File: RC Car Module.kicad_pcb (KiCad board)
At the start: 2 copper layers, 45 x 45 mm, 72 parts, among them J1 USB_C_Receptacle_USB2.0_14P, J2 Conn_01x13, J3 Conn_01x09, J4 Conn_01x02, J5 Conn_01x02, J6 Conn_01x04, J7 Conn_01x02, SW1 SW_Push, SW2 SW_Push, U1 AP62401WU-7, U2 W25Q16JVUXIQ TR, U3 RT6154AGQW, U4 TB6612FNG, U5 RP2040, Y1 12 MHz

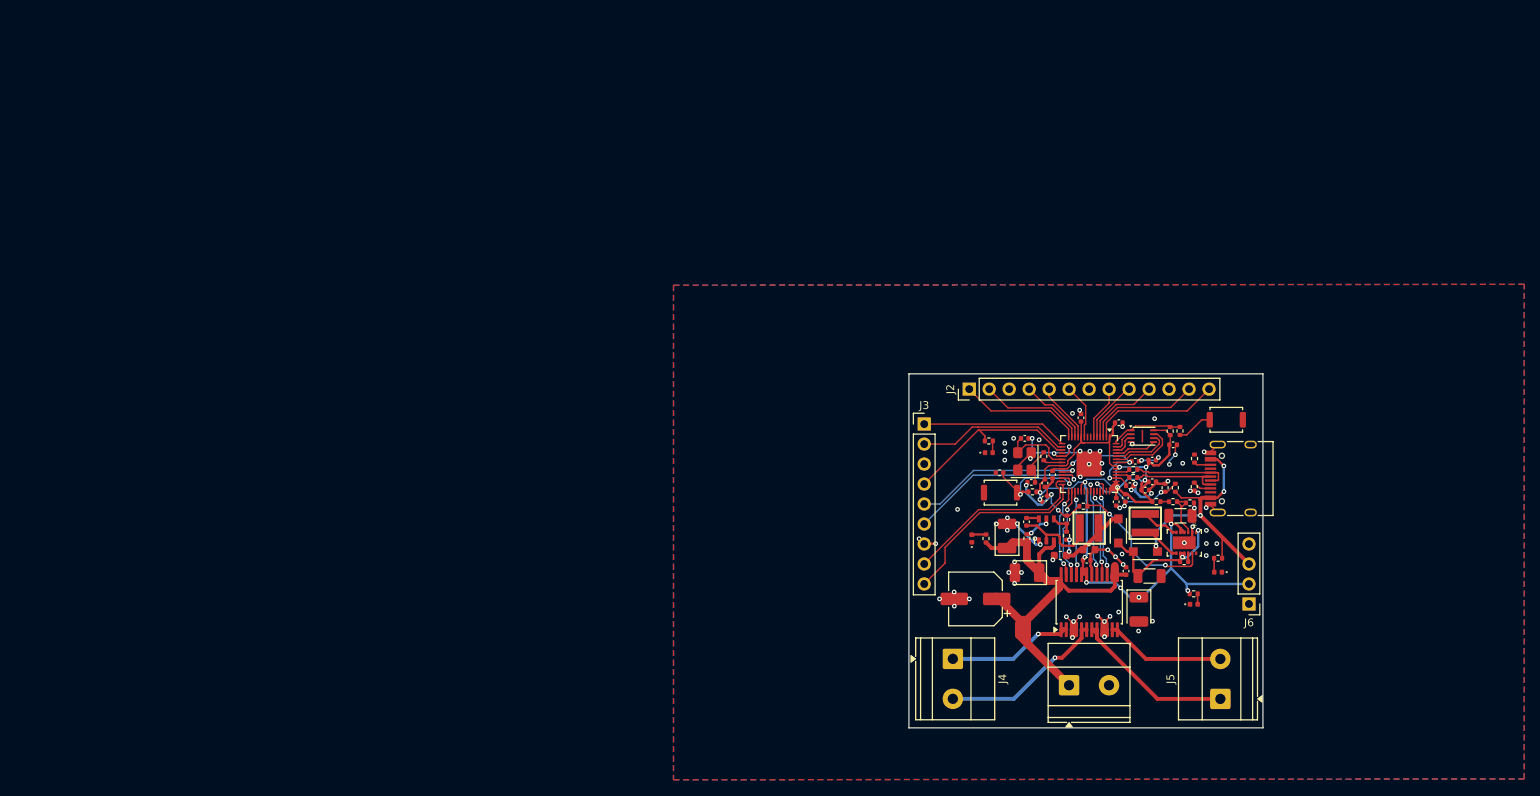
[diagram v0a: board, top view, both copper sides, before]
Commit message: Update Readme
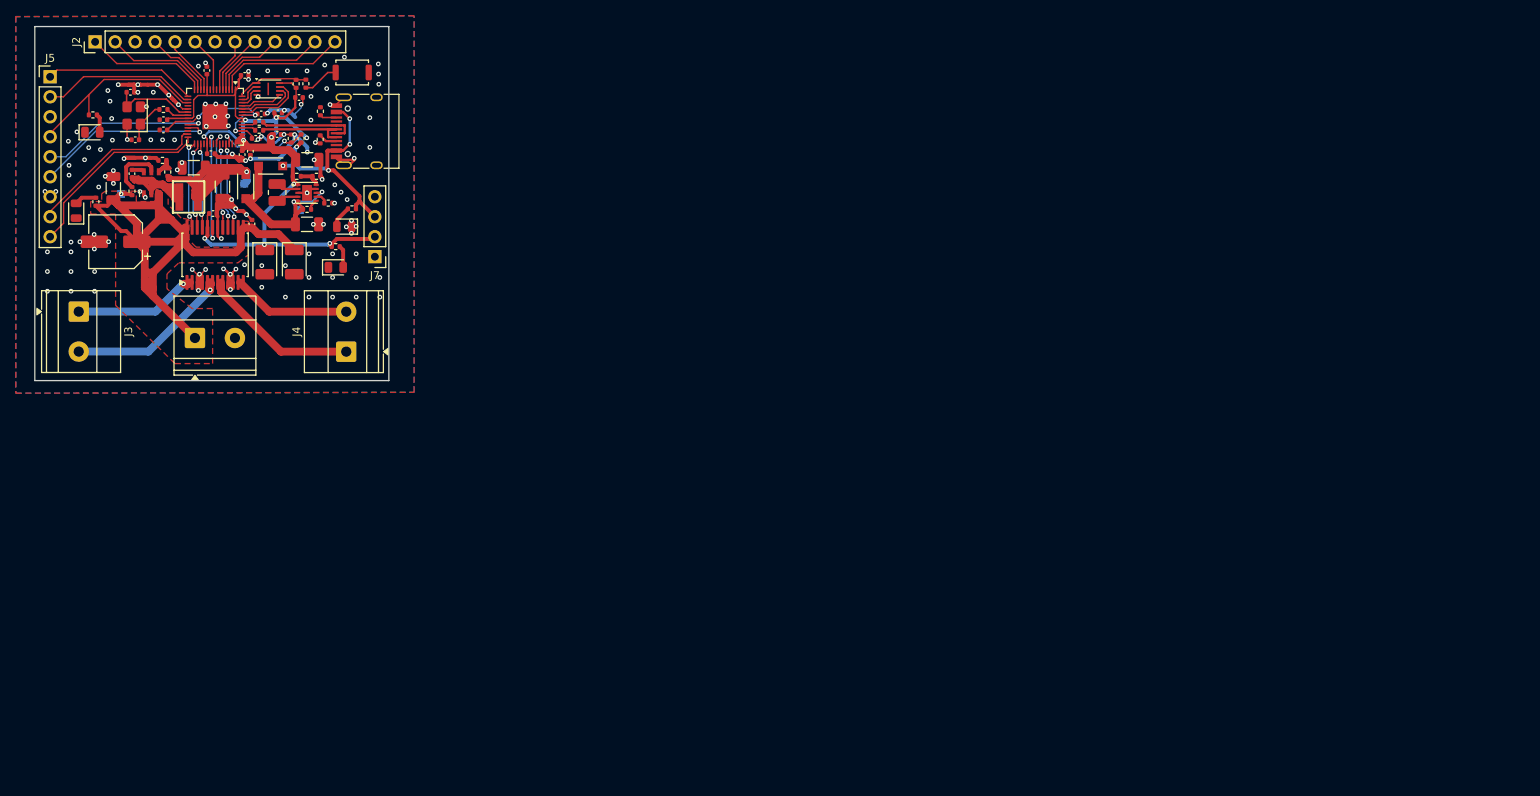
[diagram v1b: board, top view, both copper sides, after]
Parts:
- removed the C15 at (156.4, 76.3)
- removed the C23 at (155.4, 79.3)
- removed the C24 at (155.4, 77.3)
- removed C27: 0.1uF, Capacitor_SMD:C_0402_1005Metric
- removed the R12 at (171.7, 79.7)
- removed the R15 at (160.3, 80.3)
- removed the R16 at (153.8, 78.5)
- removed SW2: SW_Push, Button_Switch_SMD:SW_Push_SPST_NO_Alps_SKRK
- added C10: 1uF, Capacitor_SMD:C_0402_1005Metric, F.Cu at (55.1, 33.5)
- added C14: 0.1uF, Capacitor_SMD:C_0402_1005Metric, F.Cu at (49.4, 35.5)
- added R7: 100K, Resistor_SMD:R_0402_1005Metric, F.Cu at (61.6, 42.6)
- added TP1: TestPoint, TestPoint:TestPoint_Pad_1.0x1.0mm, B.Cu at (38.0, 40.6)
- added TP2: TestPoint, TestPoint:TestPoint_Pad_1.0x1.0mm, B.Cu at (53.7, 39.3)
- added TP3: TestPoint, TestPoint:TestPoint_Pad_1.0x1.0mm, B.Cu at (60.8, 42.7)
- C4: footprint Capacitor_Tantalum_SMD:CP_EIA-3528-15_AVX-H -> Capacitor_SMD:C_1206_3216Metric
- C6, C7: footprint Capacitor_SMD:C_0603_1608Metric -> Capacitor_SMD:C_1206_3216Metric
- C8: renamed from C9; value 47uF -> 10uF
- C9: renamed from C8; value 47uF -> 22uF
- D1, D2, D3, D4: footprint LED_SMD:LED_0402_1005Metric -> LED_SMD:LED_0805_2012Metric
- L2: footprint easyeda2kicad:IND-SMD_L4.0-W4.0_XAL4030-332MEC -> Inductor_SMD:L_1008_2520Metric
- R9: renamed from R8; value 330K -> 1.02M
- U3: value RT6154AGQW -> RT6150BGQW; footprint RP2040:QFN_4AGQW_RIT -> easyeda2kicad:WSON-10_L2.5-W2.5-P0.50-BL-EP
- moved C19 133.4 mm to (43.4, 31.2), turned to 180 degrees
- moved C11 130.9 mm to (43.4, 32.5), turned to 180 degrees
- moved C4 126.0 mm to (37.0, 39.9), turned to 90 degrees
- moved C6 123.7 mm to (47.2, 37.3), turned to 180 degrees
- moved R6 123.7 mm to (43.3, 36.3), turned to 180 degrees
- moved R2 123.2 mm to (44.0, 37.8)
- moved C13 122.1 mm to (54.5, 35.2), turned to -90 degrees
- moved U1 122.0 mm to (41.9, 39.2)
- moved R1 122.0 mm to (39.4, 40.2)
- moved C1 122.0 mm to (39.4, 38.0)
- moved L1 122.0 mm to (46.6, 41.0)
- moved C5 121.9 mm to (39.8, 33.7)
- moved C2 121.9 mm to (39.2, 27.7)
- moved 1111111111111 121.5 mm to (57.0, 37.0)
- moved Y1 121.4 mm to (39.6, 30.6)
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- renumbered 111111 to 1111111111111, 1111111 to 11111111111111, C16 to C11, C17 to C12, C18 to C13, C20 to C15, C21 to C16, C22 to C17, C25 to C20, C26 to C21, C10 to C22, C11 to C23, C12 to C24, C13 to C25, C14 to C26, J4 to J3, J5 to J4, J3 to J5, J7 to J6, J6 to J7, R9 to R10, R14 to R12, R10 to R13, R13 to R14, R17 to R15, R18 to R16, R19 to R17, R20 to R18, R21 to R19, R22 to R20, R7 to R8
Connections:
- 1111111111111 pad 1: Net-(U3-VINA) -> Net-(U3-VIN)
- 11111111111111 pad 1: Net-(U3-VINA) -> Net-(U3-VIN)
- C8 pad 1: Net-(U3-VINA) -> Net-(U3-VIN)
- J2 pad 6: GPIO7 -> GPIO6
- L2 pad 1: Net-(L2-Pad1) -> Net-(U3-LX1)
- L2 pad 2: Net-(L2-Pad2) -> Net-(U3-LX2)
- R13 pad 1: Net-(U3-VINA) -> Net-(U3-PS)
- R13 pad 2: 3V3_EN -> GND
- R9 pad 2: Net-(R12-Pad1) -> Net-(U3-FB)
- U3 pad 1: Net-(U3-VINA) -> +3V3
- U3 pad 10: Net-(U3-VINA) -> Net-(U3-FB)
- U3 pad 11: Net-(U3-VINA) -> GND
- U3 pad 2: GND -> Net-(U3-LX2)
- U3 pad 3: Net-(U3-FB) -> GND
- U3 pad 4: +3V3 -> Net-(U3-LX1)
- U3 pad 5: +3V3 -> Net-(U3-VIN)
- U3 pad 6: Net-(L2-Pad2) -> Net-(U3-EN)
- U3 pad 7: Net-(L2-Pad2) -> Net-(U3-PS)
- U3 pad 8: Net-(L2-Pad1) -> Net-(U3-VIN)
- U3 pad 9: Net-(L2-Pad1) -> GND
- U4 pad 19: +3V3 -> STBY
- U5 pad 26: Net-(U5-RUN) -> unconnected-(U5-RUN-Pad26)
- U5 pad 34: unconnected-(U5-GPIO22-Pad34) -> STBY
- U5 pad 35: GPIO23 -> unconnected-(U5-GPIO23-Pad35)
- U5 pad 8: unconnected-(U5-GPIO6-Pad8) -> GPIO6
- U5 pad 9: GPIO7 -> unconnected-(U5-GPIO7-Pad9)
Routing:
- net +12V: track 61.5 -> 94.2 mm, vias 0 -> 1
- net VSYS: track 11.4 -> 38.2 mm, vias 2 -> 1
- net Net-(U3-VIN): track 0.00 -> 26.2 mm, vias 0 -> 2
- net GND: track 106.7 -> 132.2 mm, vias 79 -> 128
- net +3V3: track 134.6 -> 113.2 mm, vias 13 -> 10
- net GPIO23: track 21.2 -> 0.00 mm, vias 2 -> 0
- net Net-(U3-VINA): track 19.2 -> 0.00 mm, vias 2 -> 0
- net Net-(U5-RUN): track 16.0 -> 0.00 mm, vias 2 -> 0
- net STBY: track 0.00 -> 15.2 mm, vias 0 -> 2
- net GPIO6: track 0.00 -> 7.05 mm
- net GPIO7: track 7.03 -> 0.00 mm
- net VBUS: track 36.0 -> 30.1 mm, vias 4 -> 5
- net Net-(L2-Pad1): track 5.05 -> 0.00 mm
- net Net-(L2-Pad2): track 4.93 -> 0.00 mm
- net Net-(U3-FB): track 6.54 -> 2.69 mm
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- added copper zone on F.Cu, net +12V
